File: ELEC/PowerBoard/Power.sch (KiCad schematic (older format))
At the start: 8 parts, among them J1 CONN_01X08, J2 CONN_01X08, J3 Barrel_Jack, J4 XT60 Connector

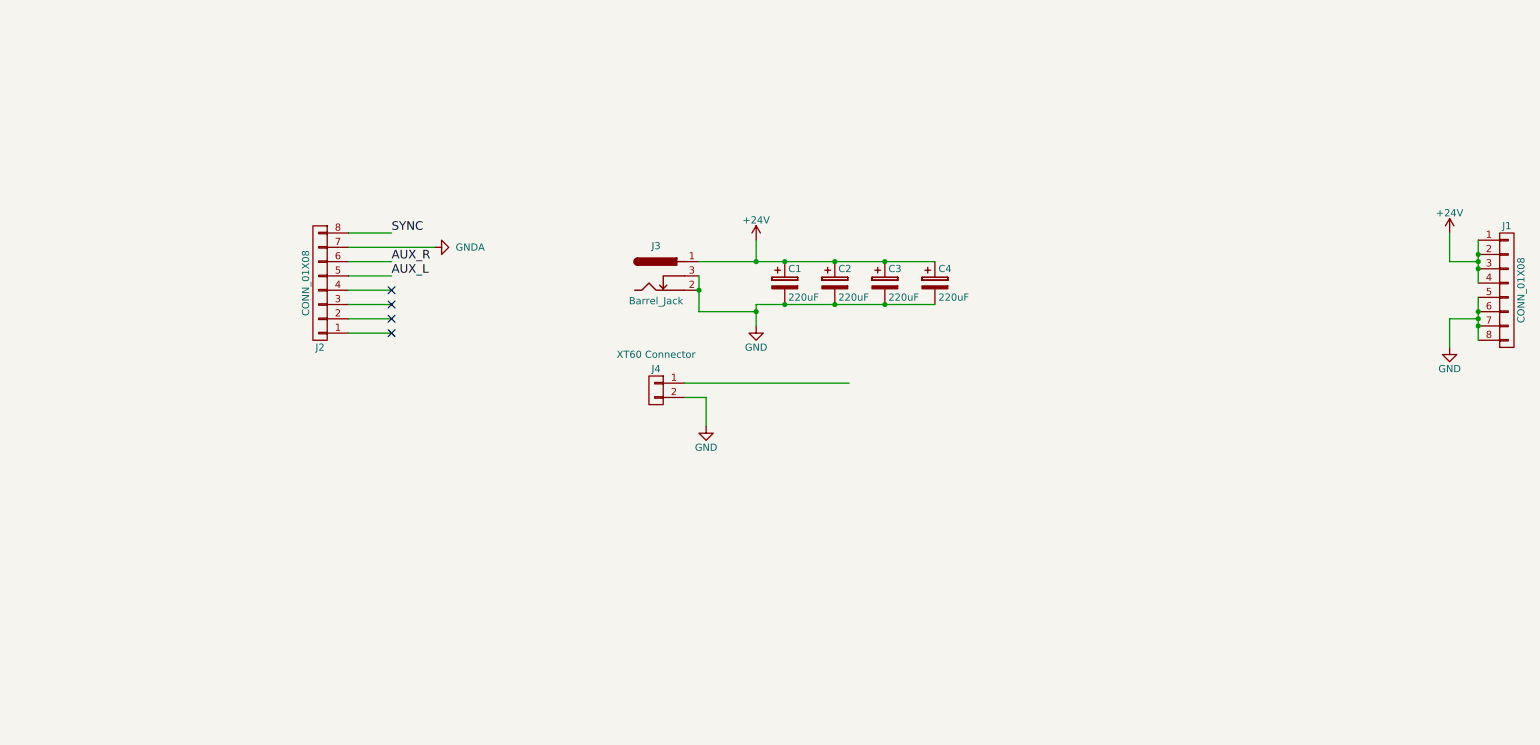
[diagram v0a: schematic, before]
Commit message: Did a whole whack on the power PCB
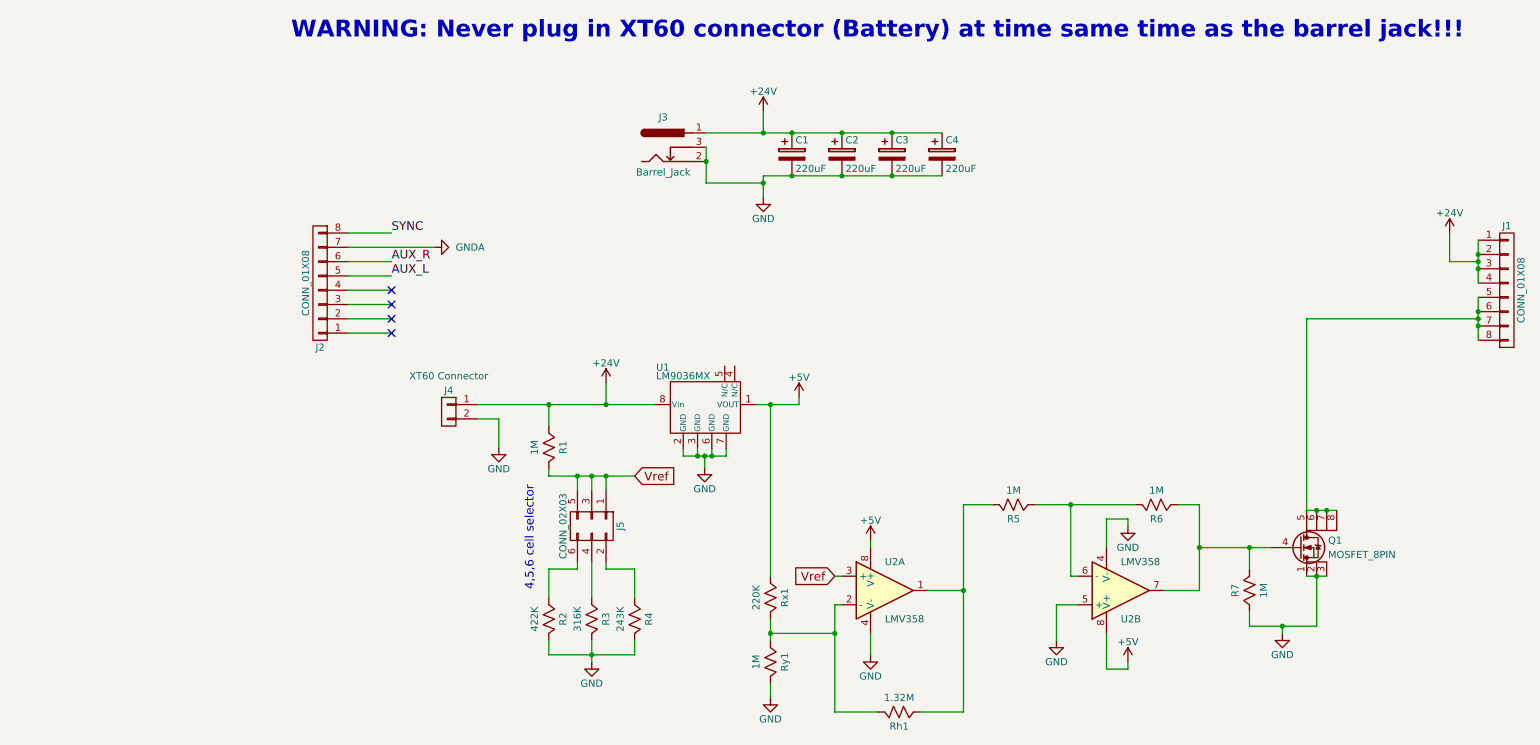
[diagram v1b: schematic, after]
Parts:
- added J5: CONN_02X03, Pin_Headers:Pin_Header_Straight_2x03_Pitch1.27mm, symbol CONN_02X03
- added Q1: MOSFET_8PIN, Housings_SOIC.pretty:SOIC-8_3.9x4.9mm_Pitch1.27mm, symbol MOSFET_8PIN
- added R1, R5, R6, R7, Ry1: 1M, Resistors_SMD:R_0805, symbol R
- added R2: 422K, Resistors_SMD:R_0805, symbol R
- added R3: 316K, Resistors_SMD:R_0805, symbol R
- added R4: 243K, Resistors_SMD:R_0805, symbol R
- added Rh1: 1.32M, Resistors_SMD:R_0805, symbol R
- added Rx1: 220K, Resistors_SMD:R_0805, symbol R
- added U1: LM9036MX, Housings_SOIC.pretty:SOIC-8_3.9x4.9mm_Pitch1.27mm, symbol LM9036MX
- added U2: LMV358, Housings_SOIC.pretty:SOIC-8_3.9x4.9mm_Pitch1.27mm, symbol LMV358
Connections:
- net labels added: +5V, Vref
- wire segments 23 -> 85
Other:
- note added: "4,5,6 cell selector"
- note added: "WARNING: Never plug in XT60 connector (Battery) at time same time as the barrel jack!!!"
- moved on the sheet: C1, C2, C3, C4, J3, J4
